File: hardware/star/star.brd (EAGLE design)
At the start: 159.7 x 163.8 mm, 520 parts, among them IC1 MAX481CSA, IC10 MAX481CSA, IC11 MAX481CSA, IC12 MAX481CSA, IC13 MAX481CSA, IC14 MAX481CSA, IC15 MAX481CSA, IC16 MAX481CSA, IC17 MAX481CSA, IC18 MAX481CSA, IC19 MAX481CSA, IC2 LD117AS12TR, IC20 MAX481CSA, IC21 MAX481CSA, IC22 LD117AS12TR, IC23 LD117AS12TR, IC3 MAX481CSA, IC4 MAX481CSA, IC5 MAX481CSA, IC6 MAX481CSA, IC7 MAX481CSA, IC8 MAX481CSA, IC9 MAX481CSA

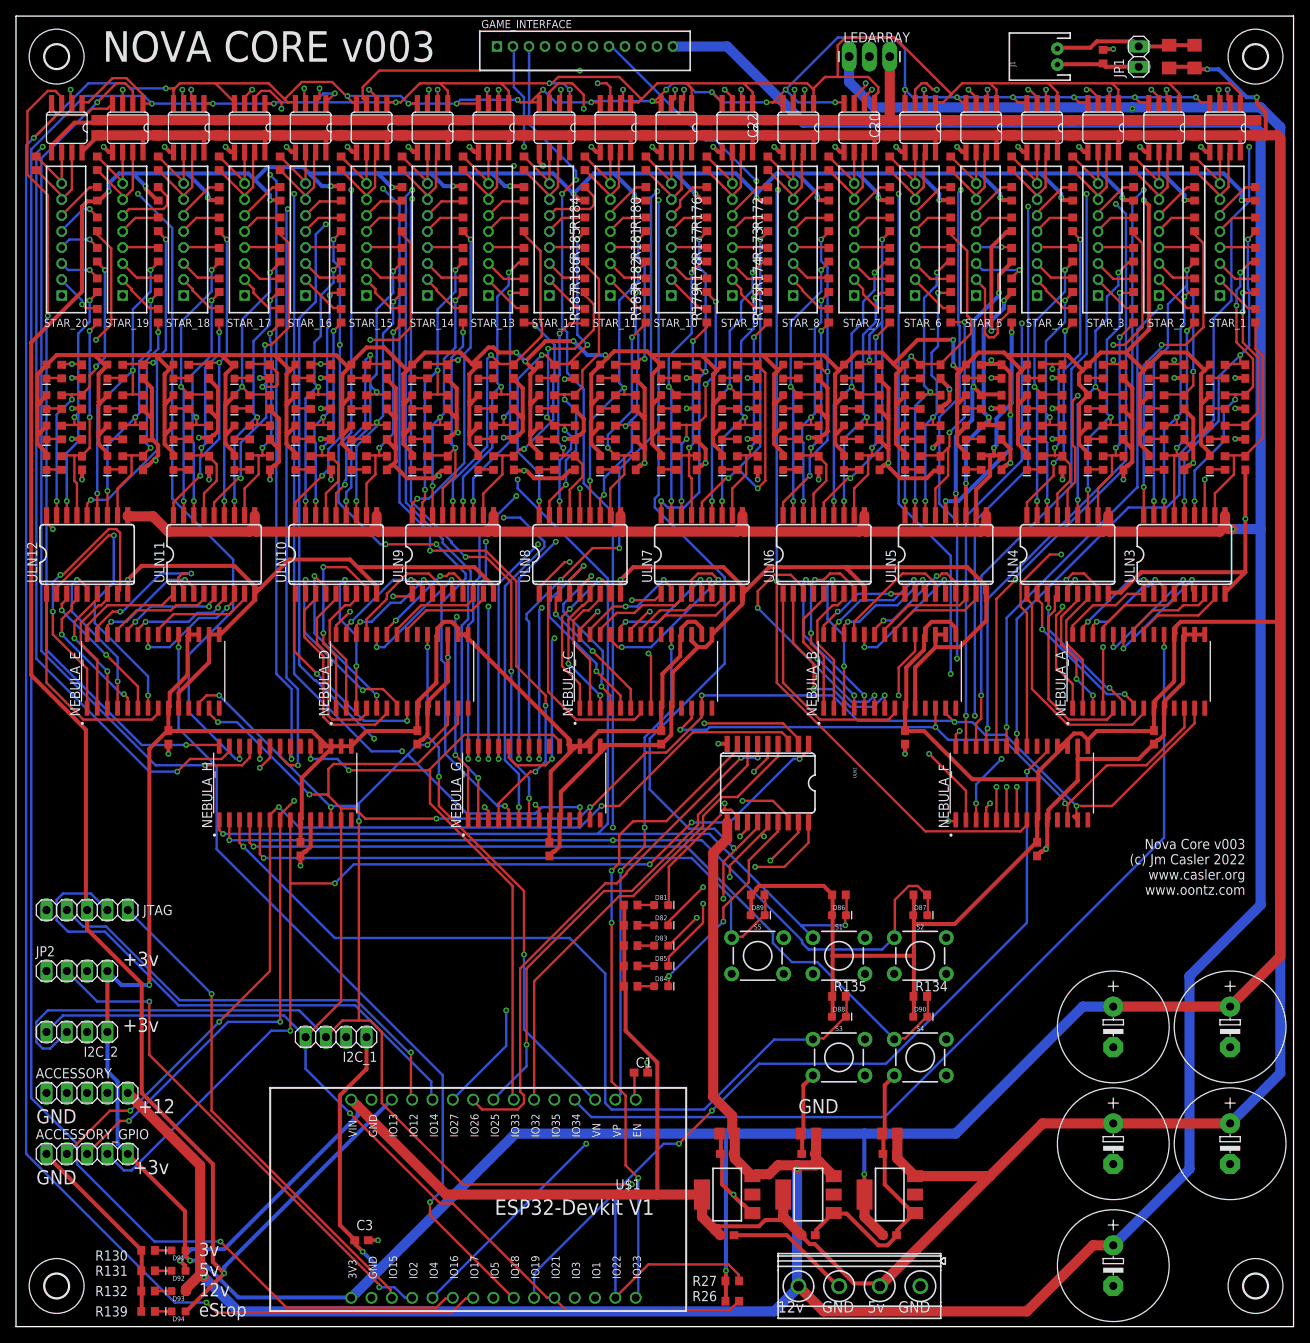
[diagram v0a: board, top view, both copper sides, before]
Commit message: Progress
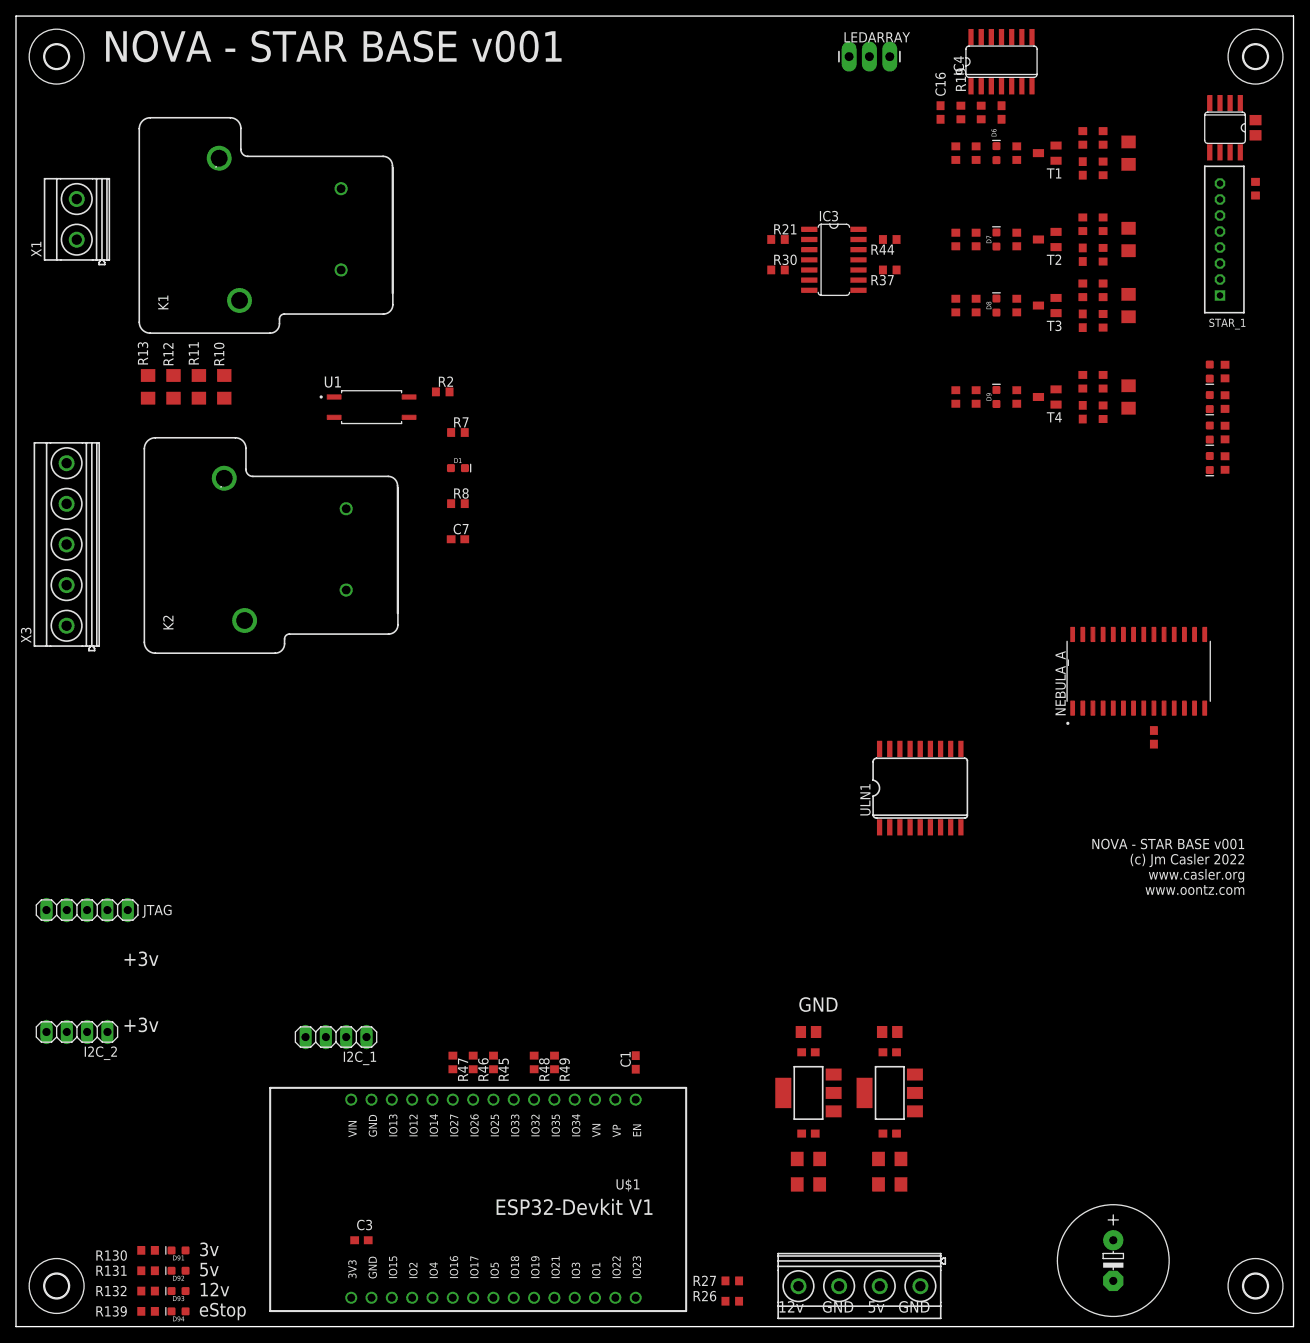
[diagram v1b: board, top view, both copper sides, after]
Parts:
- removed ACCESSORY, ACCESSORY_GPIO: (no value), pinhead:1X05
- removed C100, C101, C102, C103, C104, C105, C106, C107, C108, C109, C110, C111, C112, C113, C114, C115, C116, C117, C118, C119, C120, C121, C122, C123, C124, C37, C38, C39, C40, C41, C42, C43, C44, C45, C46, C47, C48, C49, C50, C51, C52, C53, C54, C55, C56, C57, C58, C59, C60, C61, C62, C63, C64, C65, C66, C67, C68, C73, C74, C75, C76, C77, C78, C79, C80, C81, C82, C83, C84, C85, C86, C87, C88, C93, C94, C95, C96, C97, C98, C99: 1nf, rcl:C0603
- removed C24, C25, C26, C27, C28, C29, C30, C31, C32, C33, C90: 1uf, rcl:C0805
- removed C34, C91, C92: 10uf, rcl:C0603
- removed C69, C70, C71, C72: 2200uf, rcl:E5-13
- removed D10, D11, D12, D13, D14, D15, D16, D17, D18, D19, D20, D21, D22, D23, D24, D25, D26, D27, D28, D29, D30, D31, D32, D33, D34, D35, D36, D37, D38, D39, D40, D41, D42, D43, D44, D45, D46, D47, D48, D49, D50, D51, D52, D53, D54, D55, D56, D57, D58, D59, D60, D61, D62, D63, D64, D65, D66, D67, D68, D69, D70, D71, D72, D73, D74, D75, D76, D77, D78, D79, D80: (no value), SparkFun-LED:LED-0603
- removed D81, D86: red, SparkFun-LED:LED-0603
- removed D82, D87: green, SparkFun-LED:LED-0603
- removed D83, D88: blue, SparkFun-LED:LED-0603
- removed D84, D89: white, SparkFun-LED:LED-0603
- removed D85, D90: yellow, SparkFun-LED:LED-0603
- removed GAME_INTERFACE: B12B-PH-K, con-jst-ph:B12B-PH-K
- removed IC10, IC11, IC12, IC13, IC14, IC15, IC16, IC17, IC18, IC19, IC20, IC21, IC5, IC6, IC7, IC8, IC9: MAX481CSA, maxim:SO08
- removed IC23: LD117AS12TR, v-reg:SOT223
- removed J1: (no value), SparkFun-Connectors:JST-2-PTH
- removed JP1: (no value), pinhead:1X02
- removed JP2: (no value), pinhead:1X04
- removed NEBULA_B, NEBULA_C, NEBULA_D, NEBULA_E, NEBULA_F, NEBULA_G, NEBULA_H: MCP23017-E/SO, MCP23017-E_SO:SOIC127P1030X265-28N
- removed R100, R101, R102, R133, R134, R135, R136, R137, R50, R51, R52, R53, R66, R67, R69, R70, R71, R72, R73, R74, R75, R76, R77, R78, R79, R80, R81, R82, R87, R88, R89, R90, R91, R92, R93, R94, R95, R96, R97, R98, R99: 10k, rcl:R0603
- removed R103, R104, R105, R106, R140, R141, R142, R143, R144, R145, R146, R147, R148, R149, R150, R151, R152, R153, R154, R155, R156, R157, R158, R159, R160, R161, R162, R163, R164, R165, R166, R167, R168, R169, R170, R171, R172, R173, R174, R175, R176, R177, R178, R179, R180, R181, R182, R183, R184, R185, R186, R187, R188, R189, R190, R191, R192, R193, R194, R195, R196, R197, R198, R199, R200, R201, R202, R203, R204, R205, R206, R207, R208, R209, R210, R211, R212, R213, R214, R215, R216, R217, R218, R219, R54, R55, R56, R57, R58, R59, R60, R61, R62, R63, R64, R65, R83, R84, R85, R86: 68, rcl:R0603
- removed R107, R108, R109, R110, R111, R112, R113, R114, R115, R116, R117, R118, R119, R120, R121, R122, R123, R124: 120, rcl:R0603
- removed R125, R126, R127, R128, R129: 1k, rcl:R0603
- removed R138, R68: 10, rcl:R1206
- removed S1, S2, S3, S4, S5: MOMENTARY-SWITCH-SPST-PTH-6.0MM, SparkFun-Switches:TACTILE_SWITCH_PTH_6.0MM
- removed STAR_10, STAR_11, STAR_12, STAR_13, STAR_14, STAR_15, STAR_16, STAR_17, STAR_18, STAR_19, STAR_2, STAR_20, STAR_3, STAR_4, STAR_5, STAR_6, STAR_7, STAR_8, STAR_9: B8B-PH-K, con-jst-ph:B8B-PH-K
- removed ULN10, ULN11, ULN12, ULN2, ULN3, ULN4, ULN5, ULN6, ULN7, ULN8, ULN9: (no value), SparkFun-IC-Special-Function:SO18L
- added K1, K2: T90-12VDC-TL-A, relay:JT1A-PCB
- added T1, T2, T3, T4: T_PNP_MMBT5401_CHANGJ_SOT23-BEC, JLC PCB Basic Parts_loc:SOT23
- added U1: TCLT1600, TCLT1600:SOP254P1015X230-4N
- added ULN1: (no value), SparkFun-IC-Special-Function:SO18L
- added X1: MKDSN1,5/2-5,08, con-phoenix-508:MKDSN1,5/2-5,08
- added X3: MKDSN1,5/5-5,08, con-phoenix-508:MKDSN1,5/5-5,08
- C10, C11, C12, C9: value 10uf -> C_100UF/6.3V_1206; device rcl:C0603 -> JLC PCB Basic Parts_loc:C1206
- C13: value 10uf -> C_1NF/2KV_1206; device rcl:C0603 -> JLC PCB Basic Parts_loc:C1206
- C15, C19, C21, C23: value 1uf -> C_100PF/50V_0603; device rcl:C0805 -> JLC PCB Basic Parts_loc:C0603
- C16, C17: value 1uf -> C_1NF/50V_0603; device rcl:C0805 -> JLC PCB Basic Parts_loc:C0603
- C18, C20, C22: value 1uf -> C_1NF/2KV_1206; device rcl:C0805 -> JLC PCB Basic Parts_loc:C1206
- C7: value 10uf -> C_1NF/50V_0603; device rcl:C0603 -> JLC PCB Basic Parts_loc:C0603
- D1: value (none) -> red
- D6, D7, D8, D9: value (none) -> green
- IC3: value MAX481CSA -> 74HCT08D; device maxim:SO08 -> 74xx-eu:SO14
- IC4: value MAX481CSA -> 7404D; device maxim:SO08 -> 74xx-us:SO14
- R10, R11, R12, R13: value 10k -> R_4.7K_1206; device rcl:R0603 -> JLC PCB Basic Parts_loc:R1206
- R14, R21, R23, R30, R32, R37, R39, R44: value 10k -> R_2K_0603; device rcl:R0603 -> JLC PCB Basic Parts_loc:R0603
- R15, R24, R33, R40: value 10k -> R_10R_0603; device rcl:R0603 -> JLC PCB Basic Parts_loc:R0603
- R16, R25, R34, R41: value 10k -> R_12K_0603; device rcl:R0603 -> JLC PCB Basic Parts_loc:R0603
- R17, R28, R35, R42: value 10k -> R_2.7K_0603; device rcl:R0603 -> JLC PCB Basic Parts_loc:R0603
- R18, R29, R36, R43: value 10k -> R_1K_0603; device rcl:R0603 -> JLC PCB Basic Parts_loc:R0603
- R19, R20: value 10k -> R_5.1K_0603; device rcl:R0603 -> JLC PCB Basic Parts_loc:R0603
- R2: value 120 -> R_150R_0603; device rcl:R0603 -> JLC PCB Basic Parts_loc:R0603
- R22, R31, R38, R9: value 10k -> R_7.5K_0603; device rcl:R0603 -> JLC PCB Basic Parts_loc:R0603
- R45, R46, R47, R48: value 10k -> R_6.2K_0603; device rcl:R0603 -> JLC PCB Basic Parts_loc:R0603
- R49: value 10k -> R_0R_0603; device rcl:R0603 -> JLC PCB Basic Parts_loc:R0603
- R7, R8: value 10k -> 1k
- moved R13 119.4 mm to (16.5, 117.5)
- moved R10 117.5 mm to (26.0, 117.5), turned to 90 degrees
- moved R12 116.3 mm to (19.7, 117.5), turned to 90 degrees
- moved R11 113.4 mm to (22.9, 117.5)
- moved C13 113.2 mm to (139.1, 146.7), turned to 90 degrees
- moved R2 91.0 mm to (53.3, 116.8), turned to 0 degrees
- moved R8 88.7 mm to (55.2, 102.9), turned to 0 degrees
- moved R7 88.3 mm to (55.2, 111.8), turned to 0 degrees
- moved R48 87.0 mm to (64.8, 33.0)
- moved R47 85.0 mm to (54.6, 33.0)
- moved R46 80.7 mm to (57.1, 33.0)
- moved C11 79.2 mm to (109.2, 21.0), turned to 0 degrees
- moved R45 76.5 mm to (59.7, 33.0)
- moved R49 74.9 mm to (67.3, 33.0)
- moved C23 58.9 mm to (133.3, 114.3), turned to 270 degrees
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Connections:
- removed net B0: NEBULA_B.21, ULN5.8
- removed net B1: NEBULA_B.22, ULN5.7
- removed net B10: NEBULA_B.3, ULN6.6
- removed net B11: NEBULA_B.4, ULN6.5
- removed net B12: NEBULA_B.5, ULN6.4
- removed net B13: NEBULA_B.6, ULN6.3
- removed net B14: NEBULA_B.7, ULN6.2
- removed net B15: NEBULA_B.8, ULN6.1
- removed net B2: NEBULA_B.23, ULN5.6
- removed net B3: NEBULA_B.24, ULN5.5
- removed net B4: NEBULA_B.25, ULN5.4
- removed net B5: NEBULA_B.26, ULN5.3
- removed net B6: NEBULA_B.27, ULN5.2
- removed net B7: NEBULA_B.28, ULN5.1
- removed net B8: NEBULA_B.1, ULN6.8
- removed net B9: NEBULA_B.2, ULN6.7
- removed net C0: NEBULA_C.21, ULN7.8
- removed net C1: NEBULA_C.22, ULN7.7
- removed net C10: NEBULA_C.3, ULN8.6
- removed net C11: NEBULA_C.4, ULN8.5
- removed net C12: NEBULA_C.5, ULN8.4
- removed net C13: NEBULA_C.6, ULN8.3
- removed net C14: NEBULA_C.7, ULN8.2
- removed net C15: NEBULA_C.8, ULN8.1
- removed net C2: NEBULA_C.23, ULN7.6
- removed net C3: NEBULA_C.24, ULN7.5
- removed net C4: NEBULA_C.25, ULN7.4
- removed net C5: NEBULA_C.26, ULN7.3
- removed net C6: NEBULA_C.27, ULN7.2
- removed net C7: NEBULA_C.28, ULN7.1
- removed net C8: NEBULA_C.1, ULN8.8
- removed net C9: NEBULA_C.2, ULN8.7
- removed net D0: NEBULA_D.21, ULN9.8
- removed net D1: NEBULA_D.22, ULN9.7
- removed net D10: NEBULA_D.3, ULN10.6
- removed net D11: NEBULA_D.4, ULN10.5
- removed net D12: NEBULA_D.5, ULN10.4
- removed net D13: NEBULA_D.6, ULN10.3
- removed net D14: NEBULA_D.7, ULN10.2
- removed net D15: NEBULA_D.8, ULN10.1
- removed net D2: NEBULA_D.23, ULN9.6
- removed net D3: NEBULA_D.24, ULN9.5
- removed net D4: NEBULA_D.25, ULN9.4
- removed net D5: NEBULA_D.26, ULN9.3
- removed net D6: NEBULA_D.27, ULN9.2
- removed net D7: NEBULA_D.28, ULN9.1
- removed net D8: NEBULA_D.1, ULN10.8
- removed net D9: NEBULA_D.2, ULN10.7
- removed net E0: NEBULA_E.21, ULN11.8
- removed net E1: NEBULA_E.22, ULN11.7
- removed net E10: NEBULA_E.3, ULN12.6
- removed net E11: NEBULA_E.4, ULN12.5
- removed net E12: NEBULA_E.5, ULN12.4
- removed net E13: NEBULA_E.6, ULN12.3
- removed net E14: NEBULA_E.7, ULN12.2
- removed net E15: NEBULA_E.8, ULN12.1
- removed net E2: NEBULA_E.23, ULN11.6
- removed net E3: NEBULA_E.24, ULN11.5
- removed net E4: NEBULA_E.25, ULN11.4
- removed net E5: NEBULA_E.26, ULN11.3
- removed net E6: NEBULA_E.27, ULN11.2
- removed net E7: NEBULA_E.28, ULN11.1
- removed net E8: NEBULA_E.1, ULN12.8
- removed net E9: NEBULA_E.2, ULN12.7
- removed net F0: IC1.2, NEBULA_F.21
- removed net F1: IC1.3, NEBULA_F.22
- removed net F10: IC7.2, NEBULA_F.3
- removed net F11: IC7.3, NEBULA_F.4
- removed net F12: IC8.2, NEBULA_F.5
- removed net F13: IC8.3, NEBULA_F.6
- removed net F14: IC9.2, NEBULA_F.7
- removed net F15: IC9.3, NEBULA_F.8
- removed net F2: IC3.2, NEBULA_F.23
- removed net F3: IC3.3, NEBULA_F.24
- removed net F4: IC4.2, NEBULA_F.25
- removed net F5: IC4.3, NEBULA_F.26
- removed net F6: IC5.2, NEBULA_F.27
- removed net F7: IC5.3, NEBULA_F.28
- removed net F8: IC6.2, NEBULA_F.1
- removed net F9: IC6.3, NEBULA_F.2
- removed net G0: IC10.2, NEBULA_G.21
- removed net G1: IC10.3, NEBULA_G.22
- removed net G10: IC15.2, NEBULA_G.3
- removed net G11: IC15.3, NEBULA_G.4
- removed net G12: IC16.2, NEBULA_G.5
- removed net G13: IC16.3, NEBULA_G.6
- removed net G14: IC17.2, NEBULA_G.7
- removed net G15: IC17.3, NEBULA_G.8
- removed net G2: IC11.2, NEBULA_G.23
- removed net G3: IC11.3, NEBULA_G.24
- removed net G4: IC12.2, NEBULA_G.25
- removed net G5: IC12.3, NEBULA_G.26
- removed net G6: IC13.2, NEBULA_G.27
- removed net G7: IC13.3, NEBULA_G.28
- removed net G8: IC14.2, NEBULA_G.1
- removed net G9: IC14.3, NEBULA_G.2
- removed net H0: IC18.2, NEBULA_H.21
- removed net H1: IC18.3, NEBULA_H.22
- removed net H10: D88.C, GAME_INTERFACE.4, NEBULA_H.3, R135.2, S3.1
- removed net H11: D90.C, GAME_INTERFACE.5, NEBULA_H.4, R134.2, S4.1
- removed net H12: D89.C, GAME_INTERFACE.6, NEBULA_H.5, R133.2, S5.1
- removed net H13: ACCESSORY_GPIO.2, NEBULA_H.6, ULN2.3
- removed net H14: ACCESSORY_GPIO.3, NEBULA_H.7, ULN2.2
- removed net H15: ACCESSORY_GPIO.4, NEBULA_H.8, ULN2.1
- removed net H2: IC19.2, NEBULA_H.23
- removed net H3: IC19.3, NEBULA_H.24
- removed net H4: IC20.2, NEBULA_H.25
- removed net H5: IC20.3, NEBULA_H.26
- removed net H6: IC21.2, NEBULA_H.27
- removed net H7: IC21.3, NEBULA_H.28
- removed net H8: D86.C, GAME_INTERFACE.2, NEBULA_H.1, R137.2, S1.1
- removed net H9: D87.C, GAME_INTERFACE.3, NEBULA_H.2, R136.2, S2.1
- removed net N$100: D77.C, R99.2
- removed net N$101: D78.C, R100.2
- removed net N$102: D79.C, R101.2
- removed net N$103: D80.C, R102.2
- removed net N$104: R104.2, STAR_18.6
- removed net N$105: R105.2, STAR_19.6
- removed net N$106: R106.2, STAR_20.6
- removed net N$107: R103.2, STAR_17.6
- removed net N$110: IC3.7, R2.2, STAR_2.7
- removed net N$111: IC3.6, R2.1, STAR_2.8
- removed net N$112: IC4.7, R107.2, STAR_3.7
- removed net N$113: IC4.6, R107.1, STAR_3.8
- removed net N$114: IC5.7, R108.2, STAR_4.7
- removed net N$115: IC5.6, R108.1, STAR_4.8
- removed net N$116: IC6.7, R109.2, STAR_5.7
- removed net N$117: IC6.6, R109.1, STAR_5.8
- removed net N$118: IC7.7, R110.2, STAR_6.7
- removed net N$119: IC7.6, R110.1, STAR_6.8
- removed net N$120: IC8.7, R111.2, STAR_7.7
- removed net N$121: IC8.6, R111.1, STAR_7.8
- removed net N$122: IC9.7, R112.2, STAR_8.7
- removed net N$123: IC9.6, R112.1, STAR_8.8
- removed net N$124: IC10.7, R113.2, STAR_9.7
- removed net N$125: IC10.6, R113.1, STAR_9.8
- removed net N$126: IC11.7, R114.2, STAR_10.7
- removed net N$127: IC11.6, R114.1, STAR_10.8
- removed net N$128: IC12.7, R115.2, STAR_11.7
- removed net N$129: IC12.6, R115.1, STAR_11.8
- removed net N$130: IC13.7, R116.2, STAR_12.7
- removed net N$131: IC13.6, R116.1, STAR_12.8
- removed net N$132: IC14.7, R117.2, STAR_13.7
- removed net N$133: IC14.6, R117.1, STAR_13.8
- removed net N$134: IC15.7, R118.2, STAR_14.7
- removed net N$135: IC15.6, R118.1, STAR_14.8
- removed net N$136: IC16.7, R119.2, STAR_15.7
- removed net N$137: IC16.6, R119.1, STAR_15.8
- removed net N$138: IC17.7, R120.2, STAR_16.7
- removed net N$139: IC17.6, R120.1, STAR_16.8
- removed net N$140: IC18.7, R121.2, STAR_17.7
- removed net N$141: IC18.6, R121.1, STAR_17.8
- removed net N$142: IC19.7, R122.2, STAR_18.7
- removed net N$143: IC19.6, R122.1, STAR_18.8
- removed net N$144: IC20.7, R123.2, STAR_19.7
- removed net N$145: IC20.6, R123.1, STAR_19.8
- removed net N$146: IC21.7, R124.2, STAR_20.7
- removed net N$147: IC21.6, R124.1, STAR_20.8
- removed net N$148: ACCESSORY.2, ULN2.16
- removed net N$149: ACCESSORY.3, ULN2.17
- removed net N$150: ACCESSORY.4, ULN2.18
- removed net N$151: D84.A, R129.2
- removed net N$152: D85.A, R128.2
- removed net N$153: D83.A, R127.2
- removed net N$154: D82.A, R126.2
- removed net N$155: D81.A, R125.2
- removed net N$160: C37.1, R143.1, R3.1, ULN3.11
- removed net N$161: C38.1, R142.1, R4.1, ULN3.12
- removed net N$162: C39.1, R141.1, R5.1, ULN3.13
- removed net N$163: C40.1, R140.1, R6.1, ULN3.14
- removed net N$164: C44.1, R10.1, R144.1, ULN3.18
- removed net N$165: C43.1, R145.1, R9.1, ULN3.17
- removed net N$166: C42.1, R146.1, R8.1, ULN3.16
- removed net N$167: C41.1, R147.1, R7.1, ULN3.15
- removed net N$168: R143.2, STAR_1.2
- removed net N$169: R142.2, STAR_1.3
- removed net N$170: R141.2, STAR_1.4
- removed net N$171: R140.2, STAR_1.5
- removed net N$172: R147.2, STAR_2.2
- removed net N$173: R146.2, STAR_2.3
- removed net N$174: R145.2, STAR_2.4
- removed net N$175: R144.2, STAR_2.5
- removed net N$176: R151.2, STAR_3.2
- removed net N$177: R150.2, STAR_3.3
- removed net N$178: R149.2, STAR_3.4
- removed net N$179: R148.2, STAR_3.5
- removed net N$180: R155.2, STAR_4.2
- removed net N$181: R154.2, STAR_4.3
- removed net N$182: R153.2, STAR_4.4
- removed net N$183: R152.2, STAR_4.5
- removed net N$184: C45.1, R11.1, R151.1, ULN4.11
- removed net N$185: C46.1, R12.1, R150.1, ULN4.12
- removed net N$186: C47.1, R13.1, R149.1, ULN4.13
- removed net N$187: C48.1, R14.1, R148.1, ULN4.14
- removed net N$188: C52.1, R152.1, R18.1, ULN4.18
- removed net N$189: C51.1, R153.1, R17.1, ULN4.17
- removed net N$190: C50.1, R154.1, R16.1, ULN4.16
- removed net N$191: C49.1, R15.1, R155.1, ULN4.15
- removed net N$192: C53.1, R159.1, R19.1, ULN5.11
- removed net N$193: C56.1, R156.1, R22.1, ULN5.14
- removed net N$194: C55.1, R157.1, R21.1, ULN5.13
- removed net N$195: C54.1, R158.1, R20.1, ULN5.12
- removed net N$196: C60.1, R160.1, R28.1, ULN5.18
- removed net N$197: C59.1, R161.1, R25.1, ULN5.17
- removed net N$198: C58.1, R162.1, R24.1, ULN5.16
- removed net N$199: C57.1, R163.1, R23.1, ULN5.15
- removed net N$200: R159.2, STAR_5.2
- removed net N$201: R158.2, STAR_5.3
- removed net N$202: R157.2, STAR_5.4
- removed net N$203: R156.2, STAR_5.5
- removed net N$204: R163.2, STAR_6.2
- removed net N$205: R162.2, STAR_6.3
- removed net N$206: R161.2, STAR_6.4
- removed net N$207: R160.2, STAR_6.5
- removed net N$208: R167.2, STAR_7.2
- removed net N$209: R166.2, STAR_7.3
- removed net N$210: R165.2, STAR_7.4
- removed net N$211: R164.2, STAR_7.5
- removed net N$212: R171.2, STAR_8.2
- removed net N$213: R170.2, STAR_8.3
- removed net N$214: R169.2, STAR_8.4
- removed net N$215: R168.2, STAR_8.5
- removed net N$216: C61.1, R167.1, R29.1, ULN6.11
- removed net N$217: C62.1, R166.1, R30.1, ULN6.12
- removed net N$218: C63.1, R165.1, R31.1, ULN6.13
- removed net N$219: C64.1, R164.1, R32.1, ULN6.14
- removed net N$220: C68.1, R168.1, R36.1, ULN6.18
- removed net N$221: C67.1, R169.1, R35.1, ULN6.17
- removed net N$222: C66.1, R170.1, R34.1, ULN6.16
- removed net N$223: C65.1, R171.1, R33.1, ULN6.15
- removed net N$224: R175.2, STAR_9.2
- removed net N$225: R179.2, STAR_10.2
- removed net N$226: R178.2, STAR_10.3
- removed net N$227: R174.2, STAR_9.3
- removed net N$228: R173.2, STAR_9.4
- removed net N$229: R172.2, STAR_9.5
- removed net N$230: R177.2, STAR_10.4
- removed net N$231: R176.2, STAR_10.5
- removed net N$232: R183.2, STAR_11.2
- removed net N$233: R182.2, STAR_11.3
- removed net N$234: R181.2, STAR_11.4
- removed net N$235: R180.2, STAR_11.5
- removed net N$236: R187.2, STAR_12.2
- removed net N$237: R186.2, STAR_12.3
- removed net N$238: R185.2, STAR_12.4
- removed net N$239: R184.2, STAR_12.5
- removed net N$240: C73.1, R175.1, R37.1, ULN7.11
- removed net N$241: C74.1, R174.1, R38.1, ULN7.12
- removed net N$242: C75.1, R173.1, R39.1, ULN7.13
- removed net N$243: C76.1, R172.1, R40.1, ULN7.14
- removed net N$244: R191.2, STAR_13.2
- removed net N$245: C79.1, R177.1, R43.1, ULN7.17
- removed net N$246: C78.1, R178.1, R42.1, ULN7.16
- removed net N$247: C77.1, R179.1, R41.1, ULN7.15
- removed net N$248: C81.1, R183.1, R45.1, ULN8.11
- removed net N$249: C82.1, R182.1, R46.1, ULN8.12
- removed net N$250: C83.1, R181.1, R47.1, ULN8.13
- removed net N$251: C84.1, R180.1, R48.1, ULN8.14
- removed net N$252: C80.1, R176.1, R44.1, ULN7.18
- removed net N$253: C87.1, R185.1, R51.1, ULN8.17
- removed net N$254: C86.1, R186.1, R50.1, ULN8.16
- removed net N$255: C85.1, R187.1, R49.1, ULN8.15
- removed net N$256: R190.2, STAR_13.3
- removed net N$257: R189.2, STAR_13.4
- removed net N$258: R188.2, STAR_13.5
- removed net N$259: R196.2, STAR_14.2
- removed net N$260: C88.1, R184.1, R52.1, ULN8.18
- removed net N$261: R195.2, STAR_14.3
- removed net N$262: R194.2, STAR_14.4
- removed net N$263: R193.2, STAR_14.5
- removed net N$264: R199.2, STAR_15.2
- removed net N$265: R198.2, STAR_15.3
- removed net N$266: R192.2, STAR_15.5
- removed net N$267: R197.2, STAR_15.4
- removed net N$268: R203.2, STAR_16.2
- removed net N$269: R202.2, STAR_16.3
- removed net N$270: R201.2, STAR_16.4
- removed net N$271: R200.2, STAR_16.5
- removed net N$272: R216.2, STAR_20.5
- removed net N$273: R217.2, STAR_20.4
- removed net N$274: R218.2, STAR_20.3
- removed net N$275: R219.2, STAR_20.2
- removed net N$276: R212.2, STAR_19.5
- removed net N$277: R213.2, STAR_19.4
- removed net N$278: R214.2, STAR_19.3
- removed net N$279: R215.2, STAR_19.2
- removed net N$280: R208.2, STAR_18.5
- removed net N$281: R209.2, STAR_18.4
- removed net N$282: R210.2, STAR_18.3
- removed net N$283: R211.2, STAR_18.2
- removed net N$284: R204.2, STAR_17.5
- removed net N$285: R205.2, STAR_17.4
- removed net N$286: R206.2, STAR_17.3
- removed net N$287: R207.2, STAR_17.2
- removed net N$288: C97.1, R199.1, R75.1, ULN10.11
- removed net N$289: C98.1, R198.1, R76.1, ULN10.12
- removed net N$290: C99.1, R197.1, R77.1, ULN10.13
- removed net N$291: C100.1, R192.1, R78.1, ULN10.14
- removed net N$292: C108.1, R200.1, R82.1, ULN10.18
- removed net N$293: C107.1, R201.1, R81.1, ULN10.17
- removed net N$294: C106.1, R202.1, R80.1, ULN10.16
- removed net N$295: C105.1, R203.1, R79.1, ULN10.15
- removed net N$296: C93.1, R191.1, R53.1, ULN9.11
- removed net N$297: C94.1, R190.1, R66.1, ULN9.12
- removed net N$298: C95.1, R189.1, R69.1, ULN9.13
- removed net N$299: C96.1, R188.1, R70.1, ULN9.14
- removed net N$300: C104.1, R193.1, R74.1, ULN9.18
- removed net N$301: C103.1, R194.1, R73.1, ULN9.17
- removed net N$302: C102.1, R195.1, R72.1, ULN9.16
- removed net N$303: C101.1, R196.1, R71.1, ULN9.15
- removed net N$304: C109.1, R207.1, R87.1, ULN11.11
- removed net N$305: C110.1, R206.1, R88.1, ULN11.12
- removed net N$306: C111.1, R205.1, R89.1, ULN11.13
- removed net N$307: C112.1, R204.1, R90.1, ULN11.14
- removed net N$308: C116.1, R208.1, R94.1, ULN11.18
- removed net N$309: C115.1, R209.1, R93.1, ULN11.17
- removed net N$310: C114.1, R210.1, R92.1, ULN11.16
- removed net N$311: C113.1, R211.1, R91.1, ULN11.15
- removed net N$312: C117.1, R215.1, R95.1, ULN12.11
- removed net N$313: C118.1, R214.1, R96.1, ULN12.12
- removed net N$314: C119.1, R213.1, R97.1, ULN12.13
- removed net N$315: C120.1, R212.1, R98.1, ULN12.14
- removed net N$316: C124.1, R102.1, R216.1, ULN12.18
- removed net N$317: C123.1, R101.1, R217.1, ULN12.17
- removed net N$318: C122.1, R100.1, R218.1, ULN12.16
- removed net N$319: C121.1, R219.1, R99.1, ULN12.15
- removed net N$47: D25.C, R28.2
- removed net N$48: D58.C, R76.2
- removed net N$49: D59.C, R77.2
- removed net N$50: D60.C, R78.2
- removed net N$51: D81.C, GAME_INTERFACE.7, ULN2.11
- removed net N$52: D26.C, R29.2
- removed net N$53: D27.C, R30.2
- removed net N$54: D28.C, R31.2
- removed net N$55: D29.C, R32.2
- removed net N$56: D82.C, GAME_INTERFACE.8, ULN2.12
- removed net N$57: D83.C, GAME_INTERFACE.9, ULN2.13
- removed net N$58: D85.C, GAME_INTERFACE.10, ULN2.14
- removed net N$59: D84.C, GAME_INTERFACE.11, ULN2.15
- removed net N$60: D30.C, R33.2
- removed net N$61: D31.C, R34.2
- removed net N$62: D32.C, R35.2
- removed net N$63: D33.C, R36.2
- removed net N$64: D61.C, R79.2
- removed net N$65: D62.C, R80.2
- removed net N$66: D63.C, R81.2
- removed net N$67: D64.C, R82.2
- removed net N$68: D34.C, R37.2
- removed net N$69: D35.C, R38.2
- removed net N$70: D36.C, R39.2
- removed net N$71: D37.C, R40.2
- removed net N$72: R84.2, STAR_14.6
- removed net N$73: R85.2, STAR_15.6
- removed net N$74: R86.2, STAR_16.6
- removed net N$75: R83.2, STAR_13.6
- removed net N$76: D38.C, R41.2
- removed net N$77: D39.C, R42.2
- removed net N$78: D40.C, R43.2
- removed net N$79: D41.C, R44.2
- removed net N$80: D66.C, R88.2
- removed net N$81: D67.C, R89.2
- removed net N$82: D68.C, R90.2
- removed net N$83: D69.C, R91.2
- removed net N$84: D42.C, R45.2
- removed net N$85: D43.C, R46.2
- removed net N$86: D44.C, R47.2
- removed net N$87: D45.C, R48.2
- removed net N$88: D70.C, R92.2
- removed net N$89: J1.2, JP1.2, R138.1, R68.1
- removed net N$90: D71.C, R93.2
- removed net N$91: D72.C, R94.2
- removed net N$92: D73.C, R95.2
- removed net N$93: D46.C, R49.2
- removed net N$94: D47.C, R50.2
- removed net N$95: D48.C, R51.2
- removed net N$96: D49.C, R52.2
- removed net N$97: D74.C, R96.2
- removed net N$98: D75.C, R97.2
- removed net N$99: D76.C, R98.2
- new net 120_LINE: K1.NO, X1.1
- new net 120_NEUTRAL: X1.2, X3.5
- new net BOOMER_BLOWER: C22.1, R38.1, STAR_1.2
- new net BOOMER_FUEL: C20.1, R31.1, STAR_1.3
- new net BOOMER_IGNITER: C18.1, R22.1, STAR_1.4
- new net EN_STATUS: D94.A, IC4.6
- new net EXP_ULN0: K1.1, ULN1.18
- new net EXP_ULN1: K2.1, ULN1.17
- new net EXP_ULN2: ULN1.16
- new net EXP_ULN3: ULN1.15
- new net EXP_ULN4: ULN1.14
- new net EXP_ULN5: ULN1.13
- new net EXP_ULN6: ULN1.12
- new net EXP_ULN7: ULN1.11
- new net LOCAL_EN: IC4.4, R21.1, R30.1, R37.1, R44.1, R49.1
- new net POOFER: C13.1, R9.1, STAR_1.5
- new net STAR_ENABLE: R19.1, STAR_1.6
- net +12V: now also K1.2, K2.2, R14.2, R15.2, R23.2, R24.2, R32.2, R33.2, R39.2, R40.2, ULN1.10; no longer ACCESSORY.5, C90.1, C92.1, GAME_INTERFACE.12, IC23.3, ULN10.10, ULN11.10, ULN12.10, ULN2.10, ULN3.10, ULN4.10, ULN5.10, ULN6.10, ULN7.10, ULN8.10, ULN9.10
- net +3V3: now also IC3.14, IC4.14, R2.2; no longer ACCESSORY_GPIO.5, C10.1, C13.1, C15.1, C16.1, C17.1, C18.1, C19.1, C20.1, C21.1, C22.1, C23.1, C24.1, C25.1, C26.1, C27.1, C28.1, C29.1, C30.1, C31.1, C32.1, C33.1, C34.1, C7.1, C70.+, C72.+, C9.1, D86.A, D87.A, D88.A, D89.A, D90.A, IC10.8, IC11.8, IC12.8, IC13.8, IC14.8, IC15.8, IC16.8, IC17.8, IC18.8, IC19.8, IC20.8, IC21.8, IC3.8, IC4.8, IC5.8, IC6.8, IC7.8, IC8.8, IC9.8, JP2.4, NEBULA_B.15, NEBULA_B.18, NEBULA_B.9, NEBULA_C.16, NEBULA_C.18, NEBULA_C.9, NEBULA_D.15, NEBULA_D.16, NEBULA_D.18, NEBULA_D.9, NEBULA_E.17, NEBULA_E.18, NEBULA_E.9, NEBULA_F.15, NEBULA_F.17, NEBULA_F.18, NEBULA_F.9, NEBULA_G.16, NEBULA_G.17, NEBULA_G.18, NEBULA_G.9, NEBULA_H.15, NEBULA_H.16, NEBULA_H.17, NEBULA_H.18, NEBULA_H.9, R133.1, R134.1, R135.1, R136.1, R137.1, R138.2, R68.2
- net +5V: now also C10.1, C9.1; no longer C69.+, C71.+, C91.1, D1.A, D10.A, D11.A, D12.A, D13.A, D14.A, D15.A, D16.A, D17.A, D18.A, D19.A, D20.A, D21.A, D22.A, D23.A, D24.A, D25.A, D26.A, D27.A, D28.A, D29.A, D30.A, D31.A, D32.A, D33.A, D34.A, D35.A, D36.A, D37.A, D38.A, D39.A, D40.A, D41.A, D42.A, D43.A, D44.A, D45.A, D46.A, D47.A, D48.A, D49.A, D50.A, D51.A, D52.A, D53.A, D54.A, D55.A, D56.A, D57.A, D58.A, D59.A, D6.A, D60.A, D61.A, D62.A, D63.A, D64.A, D65.A, D66.A, D67.A, D68.A, D69.A, D7.A, D70.A, D71.A, D72.A, D73.A, D74.A, D75.A, D76.A, D77.A, D78.A, D79.A, D8.A, D80.A, D9.A, IC23.4, R125.1, R126.1, R127.1, R128.1, R129.1
- net 13: no longer D94.A, J1.1, JP1.1, R103.1, R104.1, R105.1, R106.1, R54.1, R55.1, R56.1, R57.1, R58.1, R59.1, R60.1, R61.1, R62.1, R63.1, R64.1, R65.1, R67.1, R83.1, R84.1, R85.1, R86.1
- net 16: no longer IC10.1, IC11.1, IC12.1, IC13.1, IC14.1, IC15.1, IC16.1, IC17.1, IC18.1, IC19.1, IC20.1, IC21.1, IC3.1, IC4.1, IC5.1, IC6.1, IC7.1, IC8.1, IC9.1
- net 17: no longer IC10.4, IC11.4, IC12.4, IC13.4, IC14.4, IC15.4, IC16.4, IC17.4, IC18.4, IC19.4, IC20.4, IC21.4, IC3.4, IC4.4, IC5.4, IC6.4, IC7.4, IC8.4, IC9.4
- net 18: no longer NEBULA_E.19
- net 19: no longer NEBULA_F.19
- net 2: no longer JP2.2
- net 21/SDA: no longer NEBULA_B.13, NEBULA_C.13, NEBULA_D.13, NEBULA_E.13, NEBULA_F.13, NEBULA_G.13, NEBULA_H.13
- net 22/SCL: no longer NEBULA_B.12, NEBULA_C.12, NEBULA_D.12, NEBULA_E.12, NEBULA_F.12, NEBULA_G.12, NEBULA_H.12
- net 23: no longer ULN2.8
- net 25: now also R45.2; no longer ULN2.7
- net 26: now also R46.2; no longer ULN2.6
- net 27: now also R47.2; no longer ULN2.5
- net 32: now also R48.2; no longer ULN2.4
- net 33: no longer NEBULA_G.19, NEBULA_H.19
- net 35: now also R49.2; no longer NEBULA_B.19
- net 36: no longer NEBULA_C.19
- net 39: no longer NEBULA_D.19
- net 5: no longer JP2.3
- net A0: now also C7.1, D1.A, R8.1, U1.3; no longer ULN3.8
- net A1: no longer ULN3.7
- net A10: now also ULN1.3; no longer ULN4.6
- net A11: now also ULN1.4; no longer ULN4.5
- net A12: now also ULN1.5; no longer ULN4.4
- net A13: now also ULN1.6; no longer ULN4.3
- net A14: now also ULN1.7; no longer ULN4.2
- net A15: now also ULN1.8; no longer ULN4.1
- net A2: no longer ULN3.6
- net A3: no longer ULN3.5
- net A4: no longer ULN3.4
- net A5: no longer ULN3.3
- net A6: now also IC1.3; no longer ULN3.2
- net A7: now also IC1.2; no longer ULN3.1
- net A8: now also ULN1.1; no longer ULN4.8
- net A9: now also ULN1.2; no longer ULN4.7
- net GND: now also D6.C, D7.C, D8.C, D9.C, IC3.7, IC4.7, R18.1, R29.1, R36.1, R43.1, R7.2, R8.2, ULN1.9; no longer ACCESSORY.1, ACCESSORY_GPIO.1, C100.2, C101.2, C102.2, C103.2, C104.2, C105.2, C106.2, C107.2, C108.2, C109.2, C110.2, C111.2, C112.2, C113.2, C114.2, C115.2, C116.2, C117.2, C118.2, C119.2, C120.2, C121.2, C122.2, C123.2, C124.2, C24.2, C25.2, C26.2, C27.2, C28.2, C29.2, C30.2, C31.2, C32.2, C33.2, C34.2, C37.2, C38.2, C39.2, C40.2, C41.2, C42.2, C43.2, C44.2, C45.2, C46.2, C47.2, C48.2, C49.2, C50.2, C51.2, C52.2, C53.2, C54.2, C55.2, C56.2, C57.2, C58.2, C59.2, C60.2, C61.2, C62.2, C63.2, C64.2, C65.2, C66.2, C67.2, C68.2, C69.-, C70.-, C71.-, C72.-, C73.2, C74.2, C75.2, C76.2, C77.2, C78.2, C79.2, C80.2, C81.2, C82.2, C83.2, C84.2, C85.2, C86.2, C87.2, C88.2, C90.2, C91.2, C92.2, C93.2, C94.2, C95.2, C96.2, C97.2, C98.2, C99.2, GAME_INTERFACE.1, IC10.5, IC11.5, IC12.5, IC13.5, IC14.5, IC15.5, IC16.5, IC17.5, IC18.5, IC19.5, IC20.5, IC21.5, IC23.1, IC3.5, IC4.5, IC5.5, IC6.5, IC7.5, IC8.5, IC9.5, JP2.1, NEBULA_B.10, NEBULA_B.16, NEBULA_B.17, NEBULA_C.10, NEBULA_C.15, NEBULA_C.17, NEBULA_D.10, NEBULA_D.17, NEBULA_E.10, NEBULA_E.15, NEBULA_E.16, NEBULA_F.10, NEBULA_F.16, NEBULA_G.10, NEBULA_G.15, NEBULA_H.10, R67.2, S1.3, S2.3, S3.3, S4.3, S5.3, STAR_10.1, STAR_11.1, STAR_12.1, STAR_13.1, STAR_14.1, STAR_15.1, STAR_16.1, STAR_17.1, STAR_18.1, STAR_19.1, STAR_2.1, STAR_20.1, STAR_3.1, STAR_4.1, STAR_5.1, STAR_6.1, STAR_7.1, STAR_8.1, STAR_9.1, ULN10.9, ULN11.9, ULN12.9, ULN2.9, ULN3.9, ULN4.9, ULN5.9, ULN6.9, ULN7.9, ULN8.9, ULN9.9
- net N$10: now also R10.1, R11.2; no longer R58.2, STAR_5.6
- net N$11: now also R10.2, U1.1; no longer D6.C, R7.2
- net N$12: now also D1.C, R7.1; no longer D7.C, R8.2
- net N$13: now also K2.NO, X3.2; no longer D8.C, R9.2
- net N$14: now also K1.C, X3.4; no longer D9.C, R10.2
- net N$15: now also K2.C, U1.2, X3.1; no longer R59.2, STAR_6.6
- net N$16: now also R16.2, R17.2, T1.3; no longer R60.2, STAR_7.6
- net N$17: now also C15.1, R14.1, R9.2, T1.1; no longer R61.2, STAR_8.6
- net N$18: now also D6.A, R16.1; no longer R65.2, STAR_12.6
- net N$19: now also IC3.1, R17.1, R18.2; no longer R64.2, STAR_11.6
- net N$2: now also R2.1, U1.4; no longer R55.2, STAR_2.6
- net N$20: now also R15.1, T1.2; no longer D10.C, R11.2
- net N$21: now also IC4.2, R20.1; no longer D11.C, R12.2
- net N$22: now also C17.1, IC4.3, IC4.5, R20.2; no longer D12.C, R13.2
- net N$23: now also C16.1, IC4.1, R19.2; no longer D13.C, R14.2
- net N$24: now also IC3.2, R21.2; no longer R63.2, STAR_10.6
- net N$25: now also C19.1, R22.2, R23.1, T2.1; no longer R62.2, STAR_9.6
- net N$26: now also R25.2, R28.2, T2.3; no longer D1.C, R53.2
- net N$27: now also D7.A, R25.1; no longer D50.C, R66.2
- net N$28: now also IC3.4, R28.1, R29.2; no longer D14.C, R15.2
- net N$29: now also R24.1, T2.2; no longer D15.C, R16.2
- net N$30: now also IC3.5, R30.2; no longer D16.C, R17.2
- net N$31: now also C21.1, R31.2, R32.1, T3.1; no longer D17.C, R18.2
- net N$32: now also R34.2, R35.2, T3.3; no longer D51.C, R69.2
- net N$33: now also D8.A, R34.1; no longer D52.C, R70.2
- net N$34: now also IC3.9, R35.1, R36.2; no longer D65.C, R87.2
- net N$35: now also R33.1, T3.2; no longer D53.C, R71.2
- net N$36: now also IC3.10, R37.2; no longer D18.C, R19.2
- net N$37: now also C23.1, R38.2, R39.1, T4.1; no longer D19.C, R20.2
- net N$38: now also R41.2, R42.2, T4.3; no longer D20.C, R21.2
- net N$39: now also D9.A, R41.1; no longer D21.C, R22.2
- net N$40: now also IC3.12, R42.1, R43.2; no longer D54.C, R72.2
- net N$41: now also R40.1, T4.2; no longer D55.C, R73.2
- net N$42: now also IC3.13, R44.2; no longer D56.C, R74.2
- net N$43: now also IC3.3, R45.1; no longer D57.C, R75.2
- net N$44: now also IC3.6, R46.1; no longer D22.C, R23.2
- net N$45: now also IC3.8, R47.1; no longer D23.C, R24.2
- net N$46: now also IC3.11, R48.1; no longer D24.C, R25.2
- net N$7: now also R13.1, X3.3; no longer R56.2, STAR_3.6
- net N$8: now also R12.1, R13.2; no longer R57.2, STAR_4.6
- net N$9: now also R11.1, R12.2; no longer R54.2, STAR_1.6
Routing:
- net +5V: track 935.7 -> 0.00 mm, vias 9 -> 0
- net +3V3: track 926.9 -> 0.00 mm, vias 7 -> 0
- net GND: track 836.8 -> 0.00 mm, vias 77 -> 0
- net +12V: track 614.6 -> 0.00 mm, vias 3 -> 0
- net 13: track 454.0 -> 0.00 mm, vias 21 -> 0
- net 16: track 413.4 -> 0.00 mm, vias 8 -> 0
- net 17: track 409.2 -> 0.00 mm, vias 21 -> 0
- net 22/SCL: track 329.5 -> 0.00 mm, vias 9 -> 0
- net 21/SDA: track 315.1 -> 0.00 mm, vias 8 -> 0
- net H10: track 225.2 -> 0.00 mm, vias 1 -> 0
- net H11: track 218.3 -> 0.00 mm, vias 1 -> 0
- net H9: track 209.8 -> 0.00 mm, vias 5 -> 0
- net H12: track 196.2 -> 0.00 mm, vias 1 -> 0
- net 4: track 195.8 -> 0.00 mm, vias 1 -> 0
- net H8: track 195.2 -> 0.00 mm, vias 4 -> 0
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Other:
- board text added: "NOVA - STAR BASE v001"
- board text added: "NOVA - STAR BASE v001 (c) Jm Casler 2022 www.casler.org www.oontz.com"
- board text removed: "*"
- board text removed: "+12"
- board text removed: "NOVA CORE v003"
- board text removed: "Nova Core v003 (c) Jm Casler 2022 www.casler.org www.oontz.com"
